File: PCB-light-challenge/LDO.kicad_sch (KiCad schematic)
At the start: 6 parts

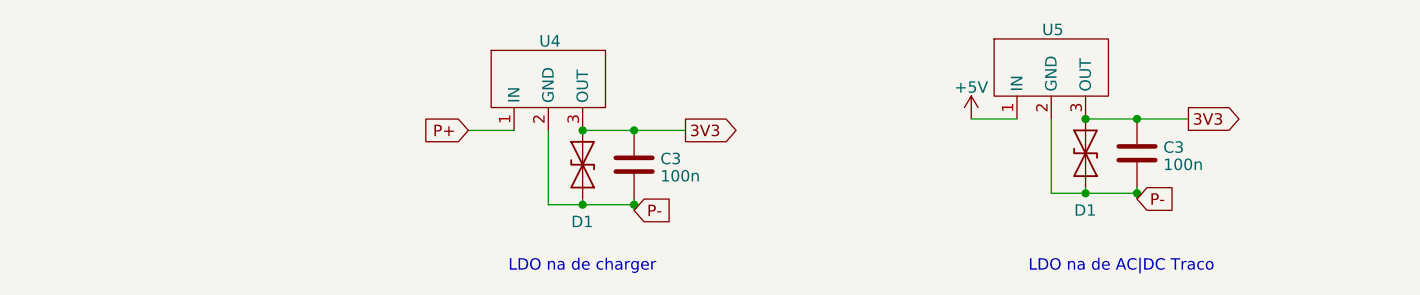
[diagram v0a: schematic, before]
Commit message: Extra caps
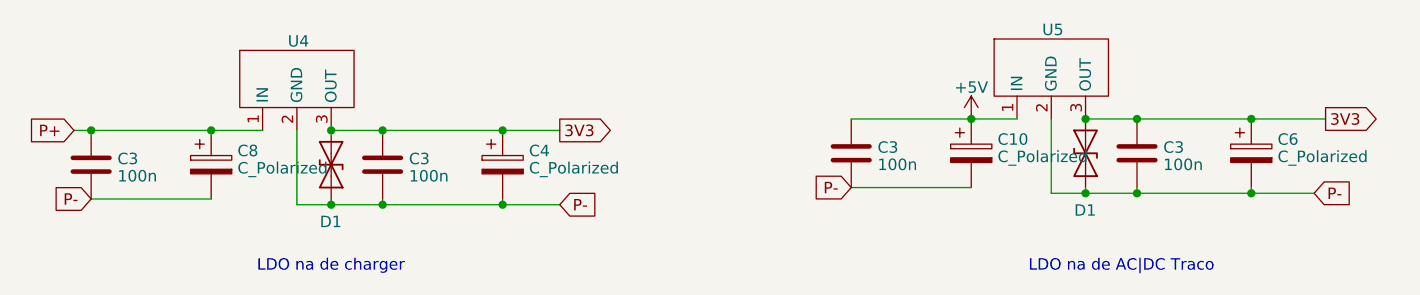
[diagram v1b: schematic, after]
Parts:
- added C10, C4, C6, C8: C_Polarized, Capacitor_THT:CP_Radial_Tantal_D5.5mm_P2.50mm, symbol Device:C_Polarized
- added C3 (x2): 100n, Capacitor_SMD:C_0603_1608Metric, symbol Device:C
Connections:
- net +5V: now also C10.1, C3.1
- net 3V3: now also C4.1, C6.1
- net P+: now also C3.1, C8.1
- net P-: now also C10.2, C3.2, C3.2, C4.2, C6.2, C8.2
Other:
- moved on the sheet: C3, D1, U4
